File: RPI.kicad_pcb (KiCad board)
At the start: 2 copper layers, 65 x 56 mm, 35 parts, among them J1 Conn_01x02_Male, J2 GPIO, J5 Conn_01x06, J6 Conn_01x04, J7 Conn_01x03, J8 Conn_01x02, J9 Conn_01x02, Q1 IRF9540N, Q2 IRF9540N, Q3 BC856BDW1, SW1 SW_SPDT, SW2 SW_SPDT, U1 LM1085-ADJ

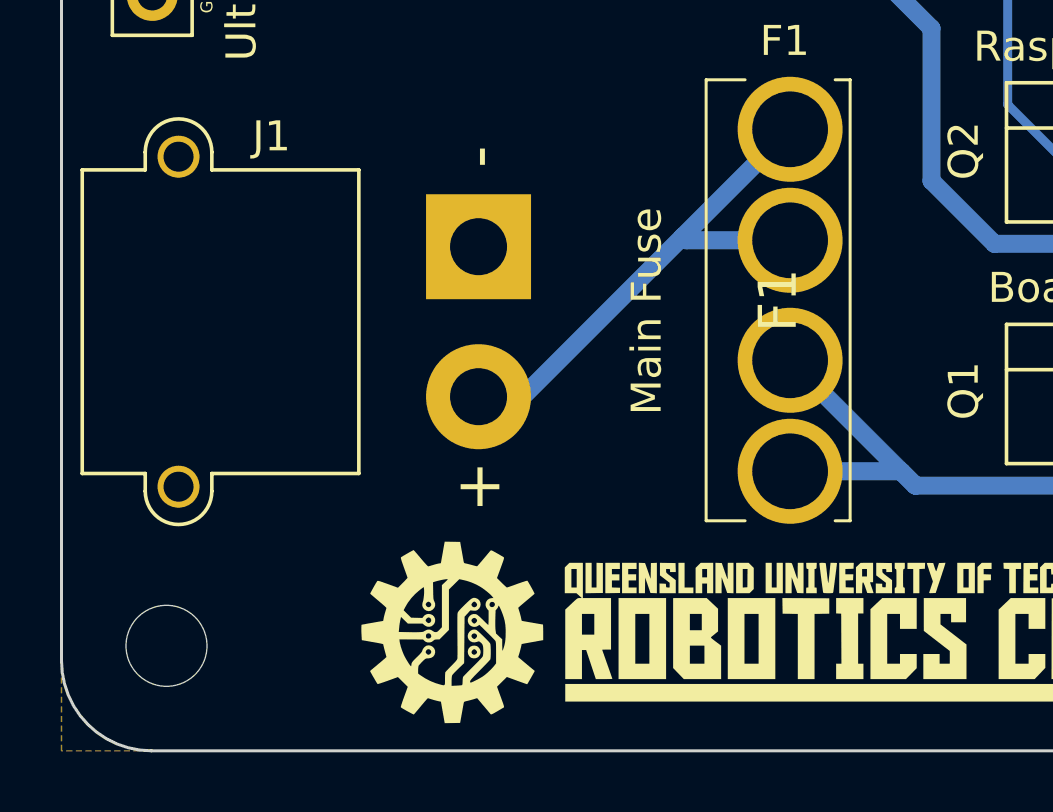
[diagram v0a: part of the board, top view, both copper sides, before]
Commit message: Finalised for a check-up
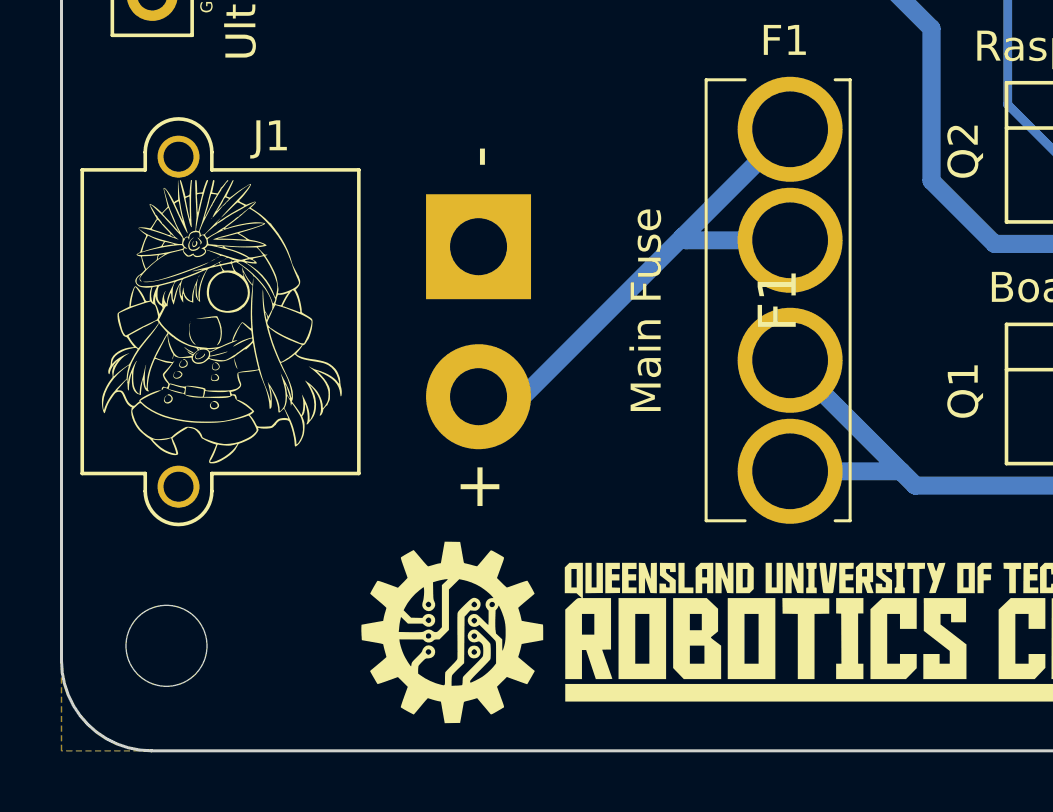
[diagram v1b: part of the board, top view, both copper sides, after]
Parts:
- added G***: LOGO, LOGO, F.Cu at (105.3, 85.7)

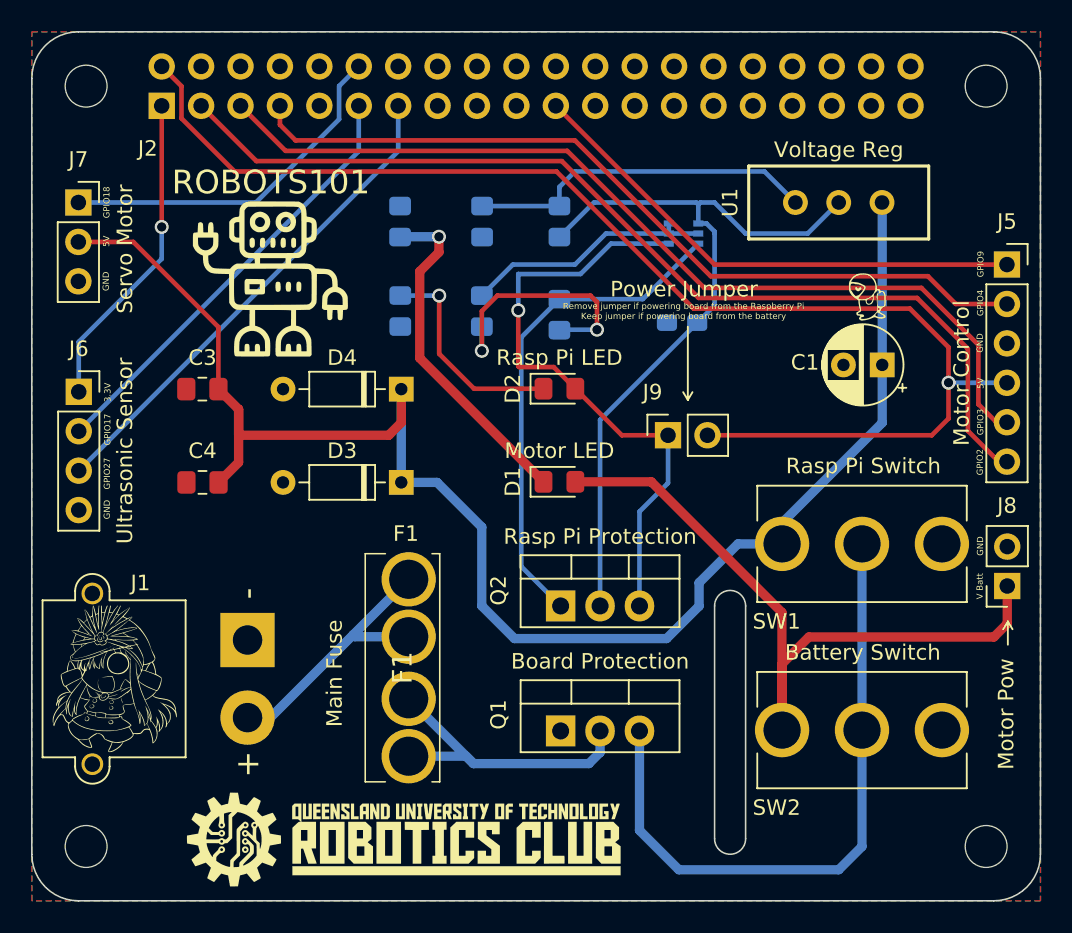
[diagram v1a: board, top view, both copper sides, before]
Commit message: Gerber files generated?
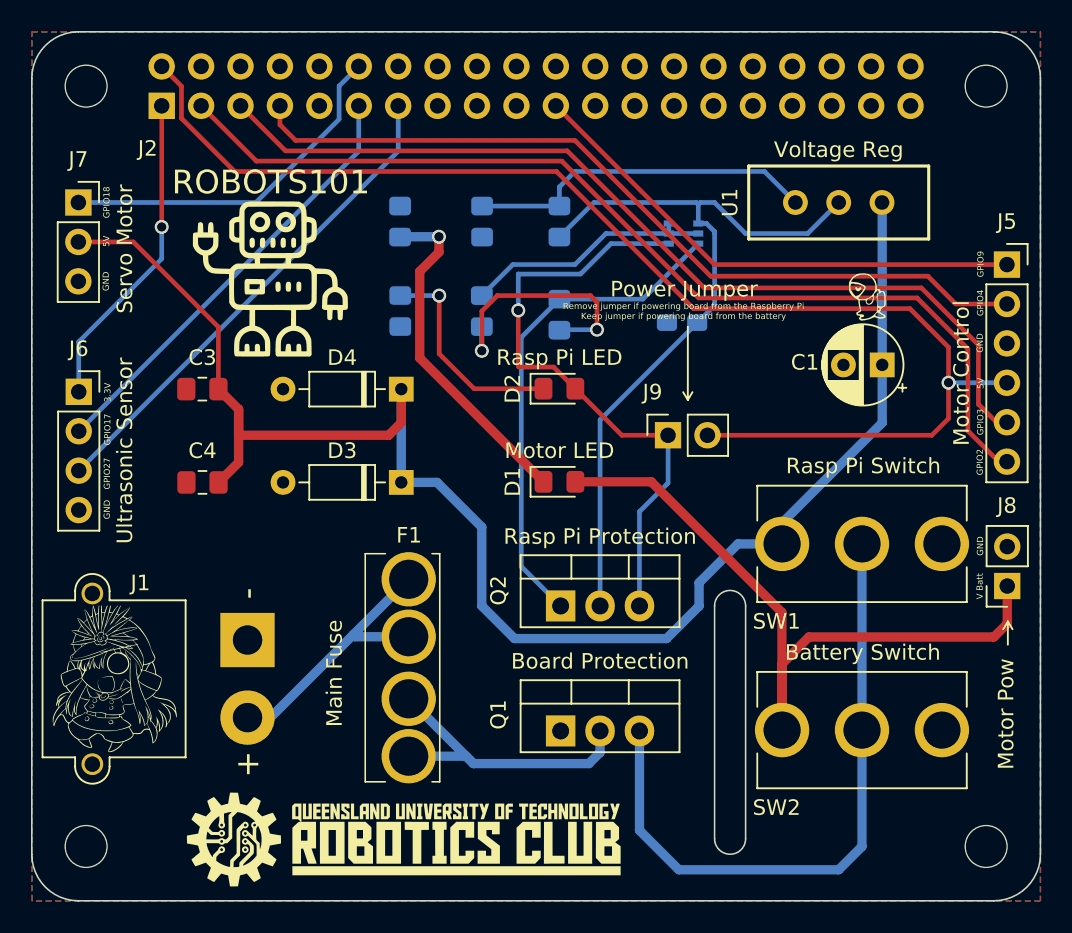
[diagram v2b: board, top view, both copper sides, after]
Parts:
- renumbered G*** to G
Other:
- board text removed: "F1"
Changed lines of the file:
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@@
   (net 6 "Net-(D2-Pad1)")
   (net 7 "VD")
-  (net 8 "Net-(J1-Pad2)")
+  (net 8 "Net-(F1-Pad1)")
   (net 9 "/GPIO2{slash}SDA1")
   (net 10 "/GPIO3{slash}SCL1")
@@
     (at 124 96.185263)
     (attr board_only exclude_from_pos_files exclude_from_bom)
-    (fp_text reference "G***" (at 2.182281 1.899801) (layer "F.SilkS")
+    (fp_text reference "G" (at 2.182281 2.814737) (layer "F.SilkS") hide
       (effects (font (size 0.3 0.3) (thickness 0.01)))
     )
@@
       (effects (font (size 1 1) (thickness 0.15)))
     )
-    (fp_text value "10u" (at 1.233747 1.783092 180) (layer "F.Fab")
+    (fp_text value "10u" (at 1.25 -3.516722 180) (layer "F.Fab")
       (effects (font (size 1 1) (thickness 0.15)))
     )
@@
     (property "Value_1" "MCCQ-122")
     (attr through_hole)
-    (fp_text reference "F1" (at 5.7 0.4 90) (layer "F.SilkS")
-      (effects (font (size 1.27 1.27) (thickness 0.254)))
+    (fp_text reference "F1" (at -2.833513 -0.019887 180) (layer "F.SilkS")
+      (effects (font (size 1 1) (thickness 0.15)))
     )
     (fp_text value "MCCQ-122" (at 5.7 0.4 90) (layer "F.SilkS") hide
       (effects (font (size 1.27 1.27) (thickness 0.254)))
     )
-    (fp_text user "${REFERENCE}" (at 5.7 0.4 90) (layer "F.Fab")
+    (fp_text user "${REFERENCE}" (at -2.618494 1.918593 180) (layer "F.Fab")
       (effects (font (size 1.27 1.27) (thickness 0.254)))
     )
@@
     (fp_line (start -1.65 -2) (end 13.05 -2) (layer "F.Fab") (width 0.2))
     (pad "1" thru_hole circle locked (at 0 0 270) (size 3.5 3.5) (drill 2.5239) (layers *.Cu *.Mask)
-      (net 8 "Net-(J1-Pad2)") (pinfunction "1") (pintype "passive"))
+      (net 8 "Net-(F1-Pad1)") (pinfunction "1") (pintype "passive"))
     (pad "2" thru_hole circle locked (at 3.7 0 270) (size 3.5 3.5) (drill 2.5239) (layers *.Cu *.Mask)
-      (net 8 "Net-(J1-Pad2)") (pinfunction "2") (pintype "passive"))
+      (net 8 "Net-(F1-Pad1)") (pinfunction "2") (pintype "passive"))
     (pad "3" thru_hole circle locked (at 7.7 0 270) (size 3.5 3.5) (drill 2.5239) (layers *.Cu *.Mask)
       (net 47 "Net-(F1-Pad3)") (pinfunction "3") (pintype "passive"))
@@
     (at 105.348613 85.695667)
     (attr board_only exclude_from_pos_files exclude_from_bom)
-    (fp_text reference "G***" (at 16.235225 12.411091) (layer "F.SilkS")
+    (fp_text reference "G" (at 0.258943 5.65) (layer "F.SilkS") hide
       (effects (font (size 0.4 0.4) (thickness 0.05)))
     )
@@
       (net 1 "GND") (pinfunction "Pin_1") (pintype "passive"))
     (pad "2" thru_hole circle (at -5 0 90) (size 3.5 3.5) (drill 1.9) (layers *.Cu *.Mask)
-      (net 8 "Net-(J1-Pad2)") (pinfunction "Pin_2") (pintype "passive"))
+      (net 8 "Net-(F1-Pad1)") (pinfunction "Pin_2") (pintype "passive"))
     (model "${KICAD6_3DMODEL_DIR}/Connector_AMASS.3dshapes/AMASS_XT30PW-M_1x02_P2.50mm_Horizontal.wrl"
       (offset (xyz 0 0 0))
@@
     (at 153.826708 61.588613)
     (attr board_only exclude_from_pos_files exclude_from_bom)
-    (fp_text reference "G***" (at -1.194086 2.150782) (layer "F.SilkS")
+    (fp_text reference "G" (at -1.826708 0.411387) (layer "F.SilkS") hide
       (effects (font (size 0.5 0.5) (thickness 0.1)))
     )
@@
     (effects (font (size 0.4 0.4) (thickness 0.08)))
   )
-  (gr_text "F1" (at 124.107573 76.340246) (layer "F.SilkS")
-    (effects (font (size 1 1) (thickness 0.15)))
-  )
   (gr_text "Motor Control" (at 159.915242 65.995222 90) (layer "F.SilkS")
